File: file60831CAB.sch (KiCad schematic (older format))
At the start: 0 parts

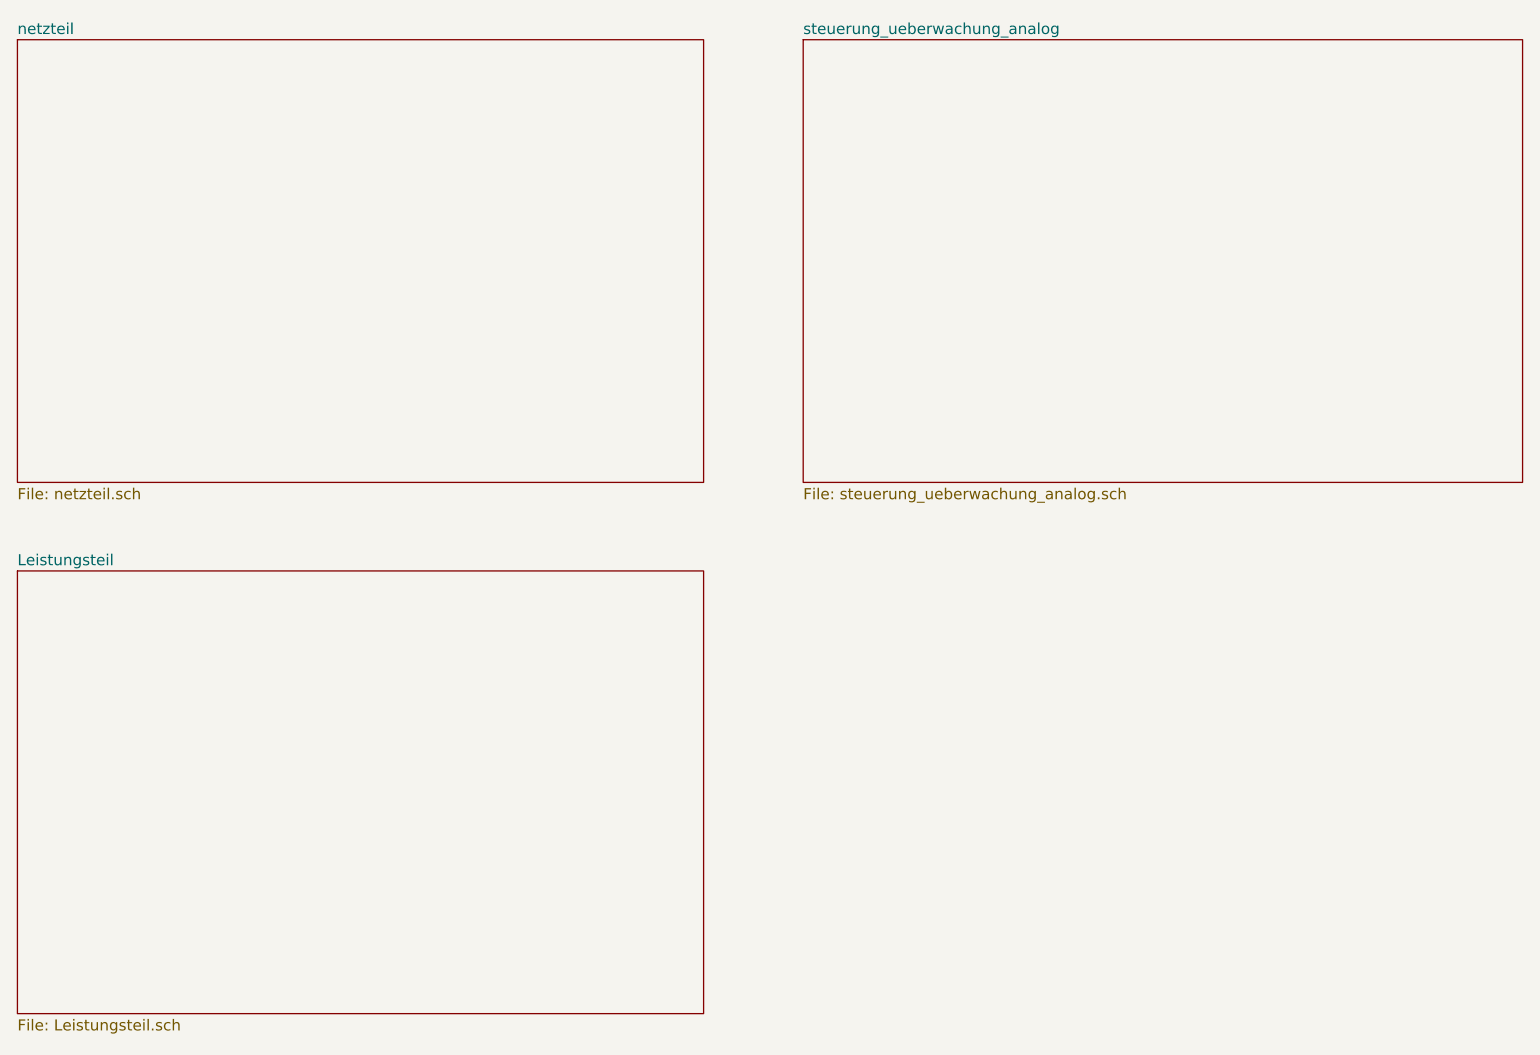
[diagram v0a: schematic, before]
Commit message: revision of Netzteil
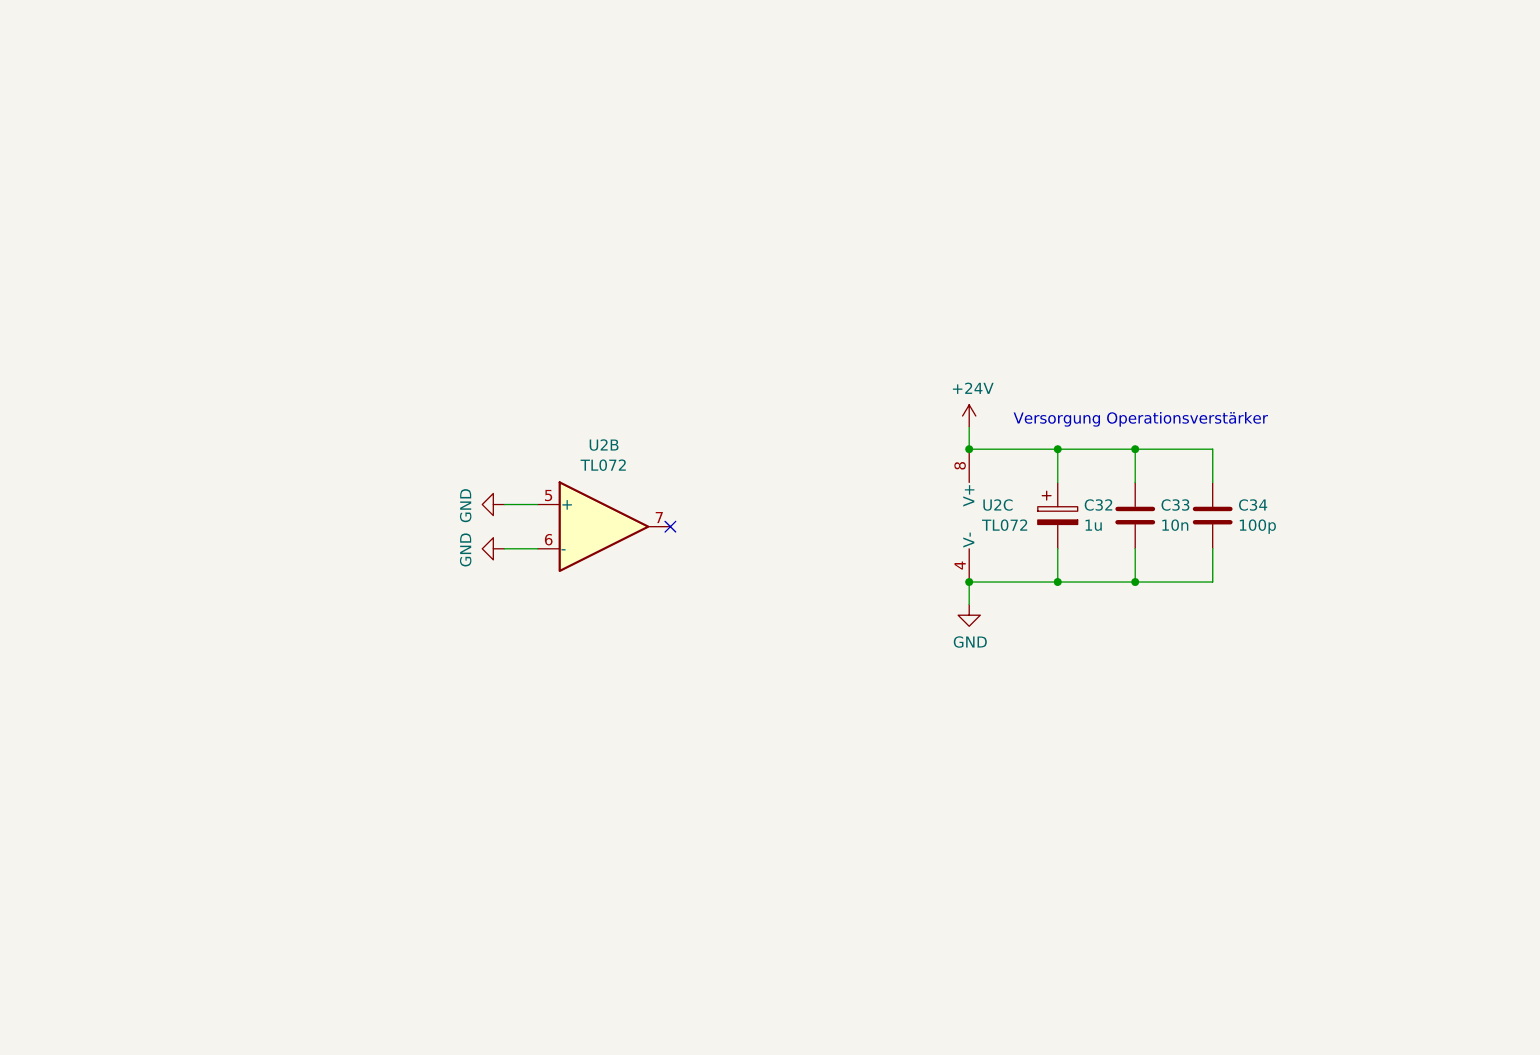
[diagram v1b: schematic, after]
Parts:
- added C32: 1u, Capacitor_THT:CP_Radial_D5.0mm_P2.50mm, symbol Device:CP
- added C33: 10n, Capacitor_THT:C_Disc_D10.0mm_W2.5mm_P5.00mm, symbol Device:C
- added C34: 100p, Capacitor_THT:C_Disc_D10.0mm_W2.5mm_P5.00mm, symbol Device:C
- added U2: TL072, symbol Amplifier_Operational:TL072
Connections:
- new net +24V: C32.1, C33.1, C34.1, U2.8 (V+)
- new net GND: C32.2, C33.2, C34.2, U2.4 (V-), U2.5 (+), U2.6 (-)
- no-connect marks 0 -> 1
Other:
- note added: "Versorgung Operationsverstärker"
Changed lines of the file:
@@
 $Descr A4 11693 8268
 encoding utf-8
-Sheet 1 7
+Sheet 3 7
 Title "Leistungsstromquelle/-senke"
 Date "01.06.2020"
@@
 Comment4 "Frank Kirschbaum"
 $EndDescr
-$Sheet
-S 900  950  3100 2000
-U 5EDECDDE
-F0 "netzteil" 50
-F1 "netzteil.sch" 50
-$EndSheet
-$Sheet
-S 4450 950  3250 2000
-U 5EDDF215
-F0 "steuerung_ueberwachung_analog" 50
-F1 "steuerung_ueberwachung_analog.sch" 50
-$EndSheet
-$Sheet
-S 900  3350 3100 2000
-U 5EE55323
-F0 "Leistungsteil" 50
-F1 "Leistungsteil.sch" 50
-$EndSheet
+$Comp
+L Amplifier_Operational:TL072 U?
+U 2 1 608458C6
+P 3550 3150
+AR Path="/5EDECDDE/608458C6" Ref="U?"  Part="2"
+AR Path="/5EDECDDE/60831CAC/608458C6" Ref="U2"  Part="2"
+F 0 "U2" H 3550 3517 50  0000 C CNN
+F 1 "TL072" H 3550 3426 50  0000 C CNN
+F 2 "" H 3550 3150 50  0001 C CNN
+F 3 "http://www.ti.com/lit/ds/symlink/tl071.pdf" H 3550 3150 50  0001 C CNN
+	2    3550 3150
+	1    0    0    -1
+$EndComp
+$Comp
+L Amplifier_Operational:TL072 U?
+U 3 1 608458CC
+P 5300 3100
+AR Path="/5EDECDDE/608458CC" Ref="U?"  Part="3"
+AR Path="/5EDECDDE/60831CAC/608458CC" Ref="U2"  Part="3"
+F 0 "U2" H 5258 3146 50  0000 L CNN
+F 1 "TL072" H 5258 3055 50  0000 L CNN
+F 2 "" H 5300 3100 50  0001 C CNN
+F 3 "http://www.ti.com/lit/ds/symlink/tl071.pdf" H 5300 3100 50  0001 C CNN
+	3    5300 3100
+	1    0    0    -1
+$EndComp
+$Comp
+L Device:CP C?
+U 1 1 60848138
+P 5600 3100
+AR Path="/60848138" Ref="C?"  Part="1"
+AR Path="/5EE24869/60848138" Ref="C?"  Part="1"
+AR Path="/5EDDF215/60848138" Ref="C?"  Part="1"
+AR Path="/5EDDF215/60068EBE/60848138" Ref="C?"  Part="1"
+AR Path="/5EDECDDE/60831CAC/60848138" Ref="C32"  Part="1"
+F 0 "C32" H 5718 3146 50  0000 L CNN
+F 1 "1u" H 5718 3055 50  0000 L CNN
+F 2 "Capacitor_THT:CP_Radial_D5.0mm_P2.50mm" H 5638 2950 50  0001 C CNN
+F 3 "~" H 5600 3100 50  0001 C CNN
+	1    5600 3100
+	1    0    0    -1
+$EndComp
+Wire Wire Line
+	5600 2800 5600 2950
+Wire Wire Line
+	5600 3250 5600 3400
+$Comp
+L Device:C C?
+U 1 1 60848140
+P 5950 3100
+AR Path="/60848140" Ref="C?"  Part="1"
+AR Path="/5EE24869/60848140" Ref="C?"  Part="1"
+AR Path="/5EDDF215/60848140" Ref="C?"  Part="1"
+AR Path="/5EDDF215/60068EBE/60848140" Ref="C?"  Part="1"
+AR Path="/5EDECDDE/60831CAC/60848140" Ref="C33"  Part="1"
+F 0 "C33" H 6065 3146 50  0000 L CNN
+F 1 "10n" H 6065 3055 50  0000 L CNN
+F 2 "Capacitor_THT:C_Disc_D10.0mm_W2.5mm_P5.00mm" H 5988 2950 50  0001 C CNN
+F 3 "~" H 5950 3100 50  0001 C CNN
+	1    5950 3100
+	1    0    0    -1
+$EndComp
+$Comp
+L Device:C C?
+U 1 1 60848146
+P 6300 3100
+AR Path="/60848146" Ref="C?"  Part="1"
+AR Path="/5EE24869/60848146" Ref="C?"  Part="1"
+AR Path="/5EDDF215/60848146" Ref="C?"  Part="1"
+AR Path="/5EDDF215/60068EBE/60848146" Ref="C?"  Part="1"
+AR Path="/5EDECDDE/60831CAC/60848146" Ref="C34"  Part="1"
+F 0 "C34" H 6415 3146 50  0000 L CNN
+F 1 "100p" H 6415 3055 50  0000 L CNN
+F 2 "Capacitor_THT:C_Disc_D10.0mm_W2.5mm_P5.00mm" H 6338 2950 50  0001 C CNN
+F 3 "~" H 6300 3100 50  0001 C CNN
+	1    6300 3100
+	1    0    0    -1
+$EndComp
+Wire Wire Line
+	5950 2800 5950 2950
+Connection ~ 5600 2800
+Wire Wire Line
+	5950 3250 5950 3400
+Wire Wire Line
+	5950 3400 5600 3400
+Connection ~ 5600 3400
+Wire Wire Line
+	6300 2950 6300 2800
+Wire Wire Line
+	6300 2800 5950 2800
+Connection ~ 5950 2800
+Wire Wire Line
+	6300 3250 6300 3400
+Wire Wire Line
+	6300 3400 5950 3400
+Connection ~ 5950 3400
+Wire Wire Line
+	5600 2800 5950 2800
+Wire Wire Line
+	5200 2800 5600 2800
+Wire Wire Line
+	5200 3400 5600 3400
+Wire Wire Line
+	5200 3400 5200 3500
+$Comp
+L power:GND #PWR?
+U 1 1 6084815B
+P 5200 3500
+AR Path="/6084815B" Ref="#PWR?"  Part="1"
+AR Path="/5EE24869/6084815B" Ref="#PWR?"  Part="1"
+AR Path="/5EDDF215/6084815B" Ref="#PWR?"  Part="1"
+AR Path="/5EDDF215/60068EBE/6084815B" Ref="#PWR?"  Part="1"
+AR Path="/5EDECDDE/60831CAC/6084815B" Ref="#PWR027"  Part="1"
+F 0 "#PWR027" H 5200 3250 50  0001 C CNN
+F 1 "GND" H 5205 3327 50  0000 C CNN
+F 2 "" H 5200 3500 50  0001 C CNN
+F 3 "" H 5200 3500 50  0001 C CNN
+	1    5200 3500
+	1    0    0    -1
+$EndComp
+Wire Wire Line
+	5200 2700 5200 2800
+Text Notes 5400 2700 0    50   ~ 0
+Versorgung Operationsverstärker
+Connection ~ 5200 2800
+Connection ~ 5200 3400
+$Comp
+L power:GND #PWR?
+U 1 1 6084EDAF
+P 3100 3050
+AR Path="/6084EDAF" Ref="#PWR?"  Part="1"
+AR Path="/5EE24869/6084EDAF" Ref="#PWR?"  Part="1"
+AR Path="/5EDDF215/6084EDAF" Ref="#PWR?"  Part="1"
+AR Path="/5EDDF215/60068EBE/6084EDAF" Ref="#PWR?"  Part="1"
+AR Path="/5EDECDDE/60831CAC/6084EDAF" Ref="#PWR024"  Part="1"
+F 0 "#PWR024" H 3100 2800 50  0001 C CNN
+F 1 "GND" H 3105 2877 50  0000 C CNN
+F 2 "" H 3100 3050 50  0001 C CNN
+F 3 "" H 3100 3050 50  0001 C CNN
+	1    3100 3050
+	0    1    1    0
+$EndComp
+$Comp
+L power:GND #PWR?
+U 1 1 6084F8D6
+P 3100 3250
+AR Path="/6084F8D6" Ref="#PWR?"  Part="1"
+AR Path="/5EE24869/6084F8D6" Ref="#PWR?"  Part="1"
+AR Path="/5EDDF215/6084F8D6" Ref="#PWR?"  Part="1"
+AR Path="/5EDDF215/60068EBE/6084F8D6" Ref="#PWR?"  Part="1"
+AR Path="/5EDECDDE/60831CAC/6084F8D6" Ref="#PWR025"  Part="1"
+F 0 "#PWR025" H 3100 3000 50  0001 C CNN
+F 1 "GND" H 3105 3077 50  0000 C CNN
+F 2 "" H 3100 3250 50  0001 C CNN
+F 3 "" H 3100 3250 50  0001 C CNN
+	1    3100 3250
+	0    1    1    0
+$EndComp
+Wire Wire Line
+	3100 3050 3250 3050
+Wire Wire Line
+	3100 3250 3250 3250
+NoConn ~ 3850 3150
+$Comp
+L power:+24V #PWR026
+U 1 1 6089BFF1
+P 5200 2700
+F 0 "#PWR026" H 5200 2550 50  0001 C CNN
+F 1 "+24V" H 5215 2873 50  0000 C CNN
+F 2 "" H 5200 2700 50  0001 C CNN
+F 3 "" H 5200 2700 50  0001 C CNN
+	1    5200 2700
+	1    0    0    -1
+$EndComp
 $Bitmap
 Pos 10900 6850

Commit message: change to SMD 1206 and restructuring
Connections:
- net labels added: +15V, -5V
- net labels removed: +24V
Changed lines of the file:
@@
 Wire Wire Line
 	5200 3400 5200 3500
-$Comp
-L power:GND #PWR?
-U 1 1 6084815B
-P 5200 3500
-AR Path="/6084815B" Ref="#PWR?"  Part="1"
-AR Path="/5EE24869/6084815B" Ref="#PWR?"  Part="1"
-AR Path="/5EDDF215/6084815B" Ref="#PWR?"  Part="1"
-AR Path="/5EDDF215/60068EBE/6084815B" Ref="#PWR?"  Part="1"
-AR Path="/5EDECDDE/60831CAC/6084815B" Ref="#PWR027"  Part="1"
-F 0 "#PWR027" H 5200 3250 50  0001 C CNN
-F 1 "GND" H 5205 3327 50  0000 C CNN
-F 2 "" H 5200 3500 50  0001 C CNN
-F 3 "" H 5200 3500 50  0001 C CNN
-	1    5200 3500
-	1    0    0    -1
-$EndComp
 Wire Wire Line
 	5200 2700 5200 2800
@@
 	3100 3250 3250 3250
 NoConn ~ 3850 3150
-$Comp
-L power:+24V #PWR026
-U 1 1 6089BFF1
-P 5200 2700
-F 0 "#PWR026" H 5200 2550 50  0001 C CNN
-F 1 "+24V" H 5215 2873 50  0000 C CNN
-F 2 "" H 5200 2700 50  0001 C CNN
-F 3 "" H 5200 2700 50  0001 C CNN
-	1    5200 2700
-	1    0    0    -1
-$EndComp
 $Bitmap
 Pos 10900 6850
@@
 EndData
 $EndBitmap
+$Comp
+L power:+15V #PWR?
+U 1 1 5F2A2518
+P 5200 2700
+F 0 "#PWR?" H 5200 2550 50  0001 C CNN
+F 1 "+15V" H 5215 2873 50  0000 C CNN
+F 2 "" H 5200 2700 50  0001 C CNN
+F 3 "" H 5200 2700 50  0001 C CNN
+	1    5200 2700
+	1    0    0    -1
+$EndComp
+$Comp
+L power:-5V #PWR?
+U 1 1 5F36F35D
+P 5200 3500
+F 0 "#PWR?" H 5200 3600 50  0001 C CNN
+F 1 "-5V" H 5215 3673 50  0000 C CNN
+F 2 "" H 5200 3500 50  0001 C CNN
+F 3 "" H 5200 3500 50  0001 C CNN
+	1    5200 3500
+	-1   0    0    1
+$EndComp
 $EndSCHEMATC
